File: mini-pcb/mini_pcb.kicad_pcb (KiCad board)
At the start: 4 copper layers, 55.5 x 56.5 mm, 32 parts, among them J3 Barrel_Jack_Switch, J4 AUDIO_IN_TRS, J5 AUDIO_OUT_TRS, U1 LM1117DT-5.0, U2 OPA1664D, U3 OPA1655DBV

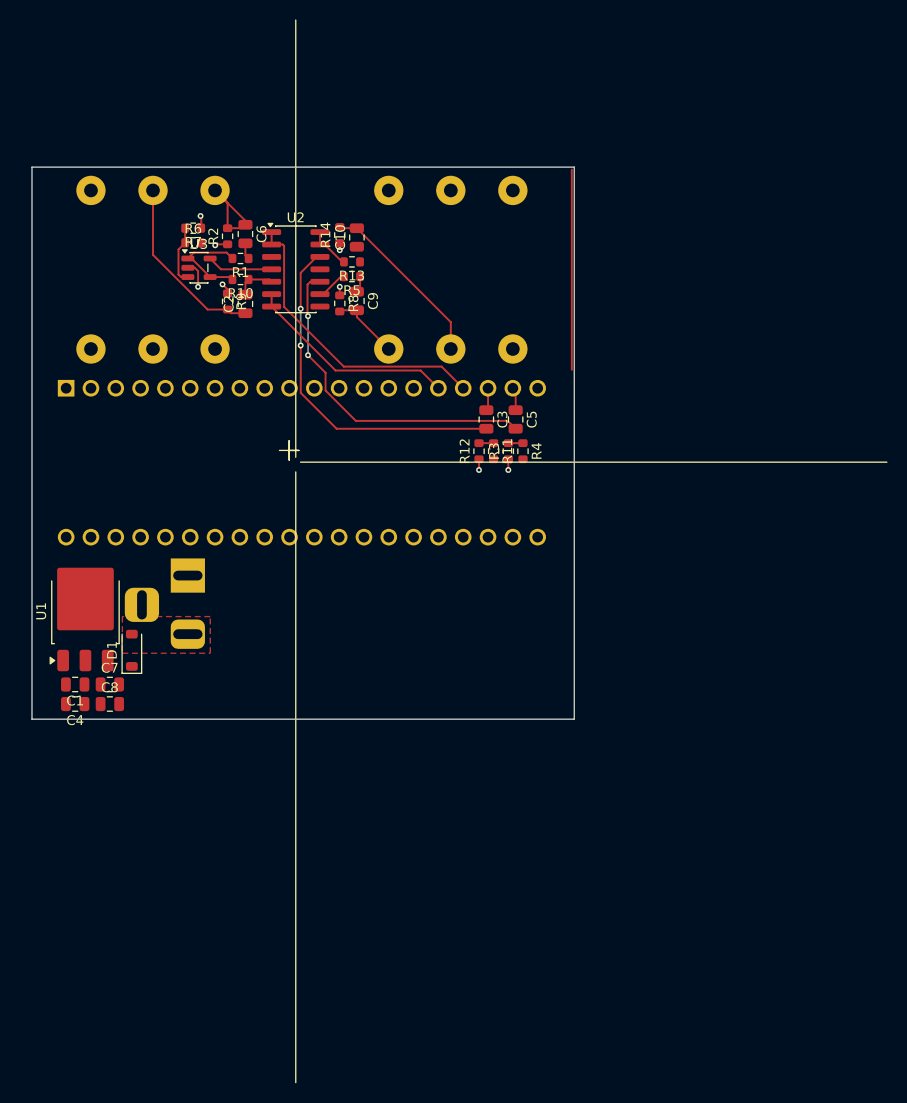
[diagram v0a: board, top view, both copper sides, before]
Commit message: pcb update
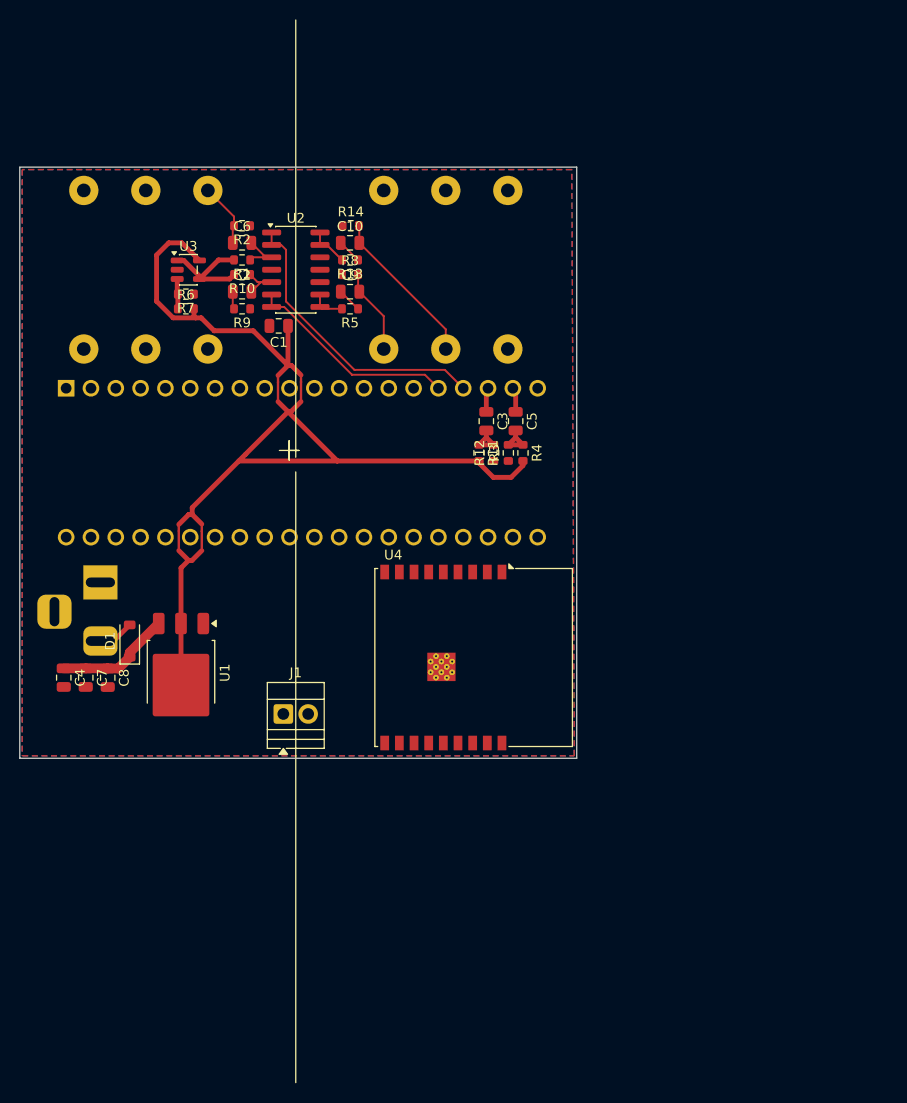
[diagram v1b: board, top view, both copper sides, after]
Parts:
- added J1: Screw_Terminal_01x02, TerminalBlock:TerminalBlock_Xinya_XY308-2.54-2P_1x02_P2.54mm_Horizontal, F.Cu at (144.7, 165.7)
- added U4: ESP32-C3-WROOM-02, RF_Module:ESP32-C3-WROOM-02, F.Cu at (161.1, 159.9)
- moved C1 42.2 mm to (144.2, 126.0)
- moved U1 11.6 mm to (134.2, 161.5), turned to -90 degrees
- moved J3 8.98 mm to (126.0, 152.2)
- moved R6 6.79 mm to (134.8, 124.2)
- moved R7 6.79 mm to (134.8, 122.8)
- moved R5 3.31 mm to (151.6, 124.2)
- moved R8 3.13 mm to (151.6, 120.8), turned to 0 degrees
- moved C4 2.94 mm to (122.2, 162.0), turned to -90 degrees
- moved C8 2.70 mm to (126.8, 162.0), turned to -90 degrees
- moved C7 2.57 mm to (124.5, 162.0), turned to -90 degrees
- moved R2 1.83 mm to (140.5, 115.8), turned to 180 degrees
- moved R9 1.66 mm to (140.5, 124.2), turned to 180 degrees
- moved R11 1.51 mm to (164.8, 139.0)
- moved R12 1.51 mm to (166.2, 139.0)
- moved R14 1.47 mm to (151.6, 115.8), turned to 0 degrees
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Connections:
- A1 pad 28: unconnected-(A1-ADC_6-Pad28) -> Net-(A1-ADC_6)
- J4 pad S: GND -> GNDA
- J5 pad S: GND -> GNDA
- R12 pad 1: DGND -> AGND
- R14 pad 1: DGND -> AGND
- R2 pad 1: DGND -> AGND
- R3 pad 1: DGND -> AGND
- R7 pad 1: DGND -> AGND
- R8 pad 1: DGND -> AGND
- R9 pad 1: DGND -> AGND
- U3 pad 2: DGND -> AGND
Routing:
- net +5V: track 6.75 -> 120.9 mm
- net Net-(U2D-+): track 37.0 -> 4.35 mm, vias 2 -> 0
- net Net-(U2C-+): track 35.6 -> 4.35 mm, vias 2 -> 0
- net AUDIO_IN_JACK_RIGHT: track 55.1 -> 38.4 mm
- net +9V: track 0.00 -> 11.9 mm
- net DGND: track 10.3 -> 0.00 mm, vias 8 -> 0
- net AUDIO_IN_JACK_LEFT: track 11.2 -> 6.52 mm
- net POWER_JACK_PWR: track 0.00 -> 3.68 mm
- net Net-(U2A-+): track 1.68 -> 5.00 mm
- net Net-(U3-+): track 6.10 -> 3.08 mm
- net Net-(C10-Pad1): track 0.00 -> 2.50 mm
- net AUDIO_OUT_JACK_RIGHT: track 18.1 -> 16.3 mm
- net AUDIO_OUT_JACK_LEFT: track 7.12 -> 8.70 mm
- net Net-(U2B-+): track 4.14 -> 5.00 mm
- net Net-(C9-Pad1): track 1.68 -> 2.50 mm
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- added copper zone on B.Cu, net AGND
- added copper zone on F.Cu, net AGND
- removed copper zone on F.Cu, net POWER_JACK_PWR
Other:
- board size 55.5 x 56.5 mm -> 57 x 60.5 mm
